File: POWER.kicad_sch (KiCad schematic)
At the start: 39 parts, among them IC1 MP1584EN, IC2 MP1584EN, J7 Conn_Jack-DC

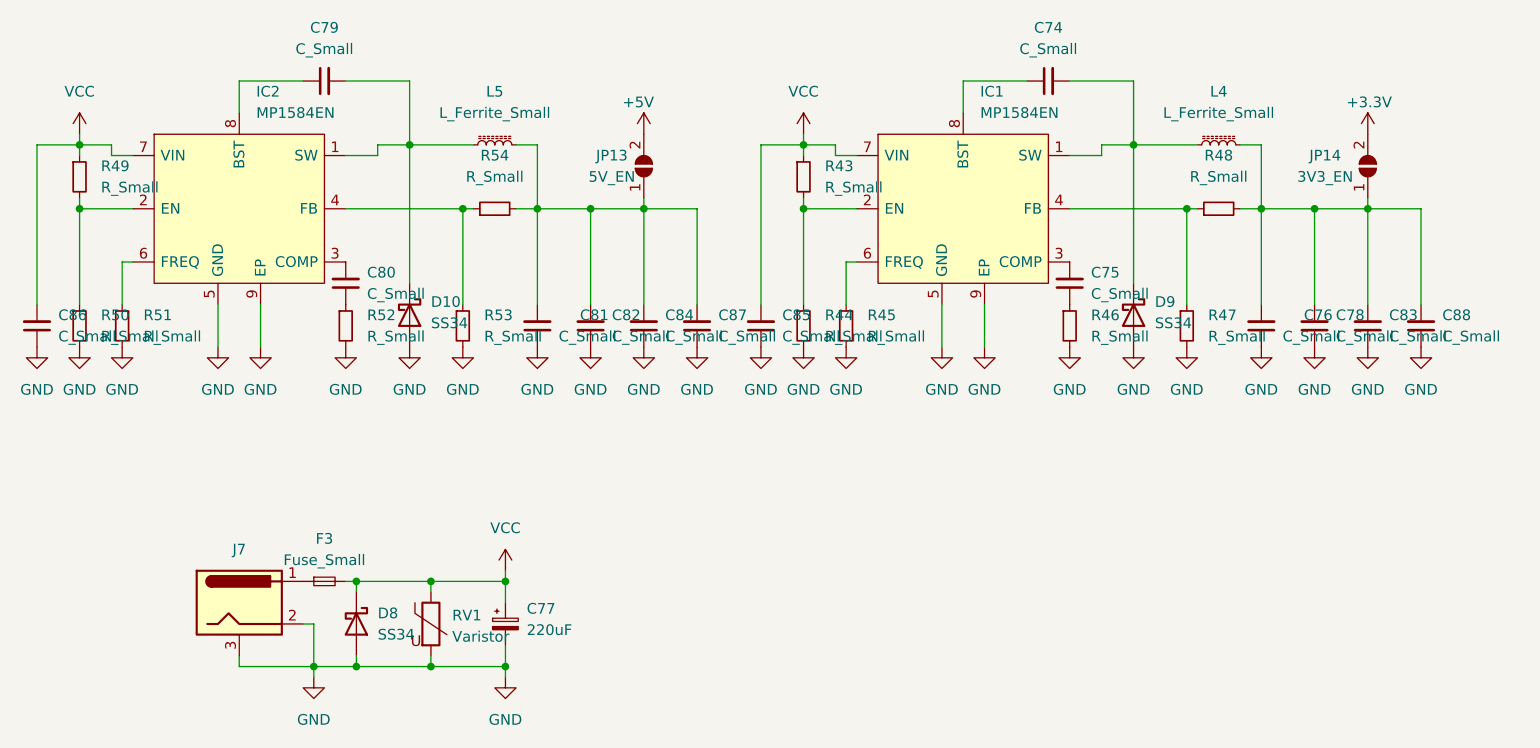
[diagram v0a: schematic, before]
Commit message: Only 1 wire to complete.
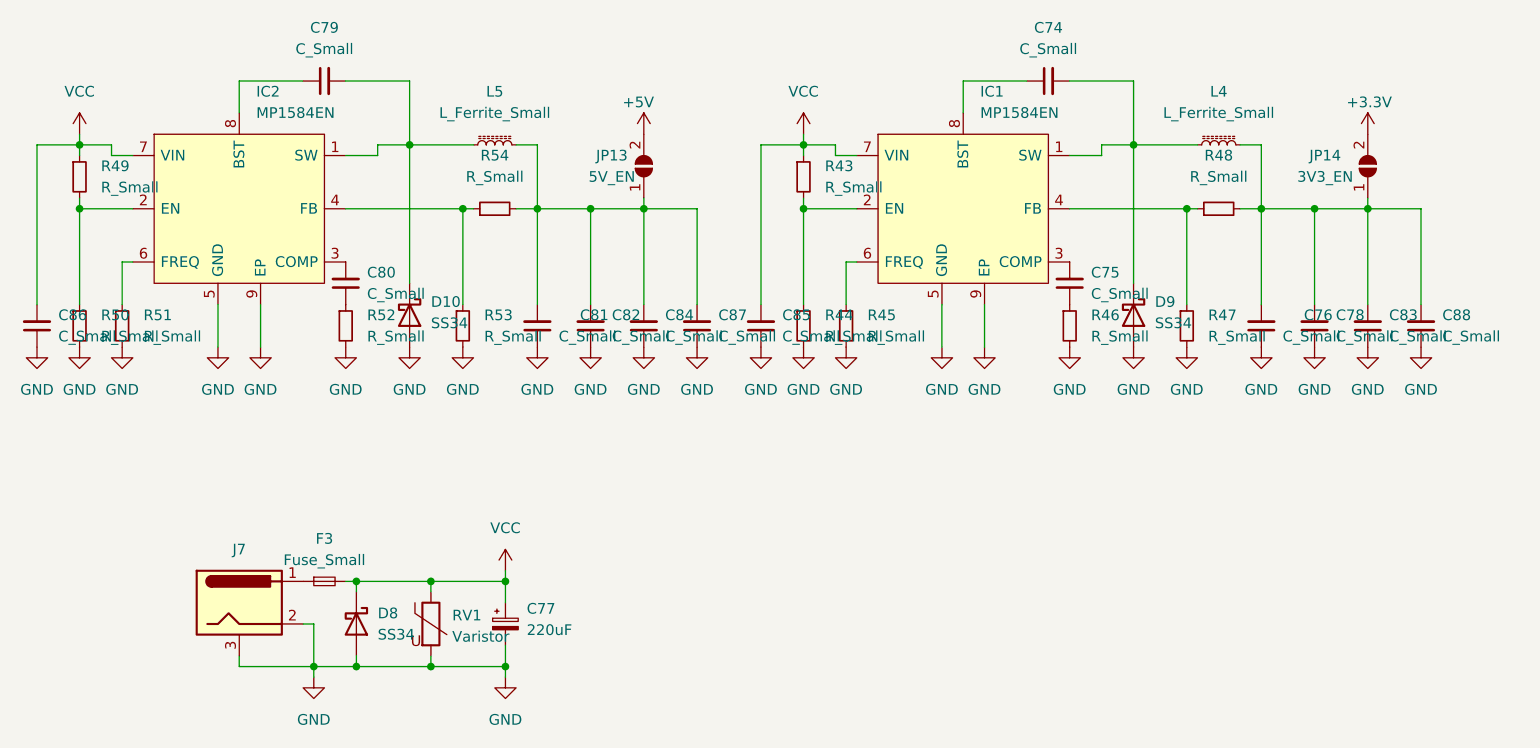
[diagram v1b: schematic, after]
